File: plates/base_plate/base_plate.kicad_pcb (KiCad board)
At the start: 2 copper layers, 135.6 x 97.4 mm, 0 parts

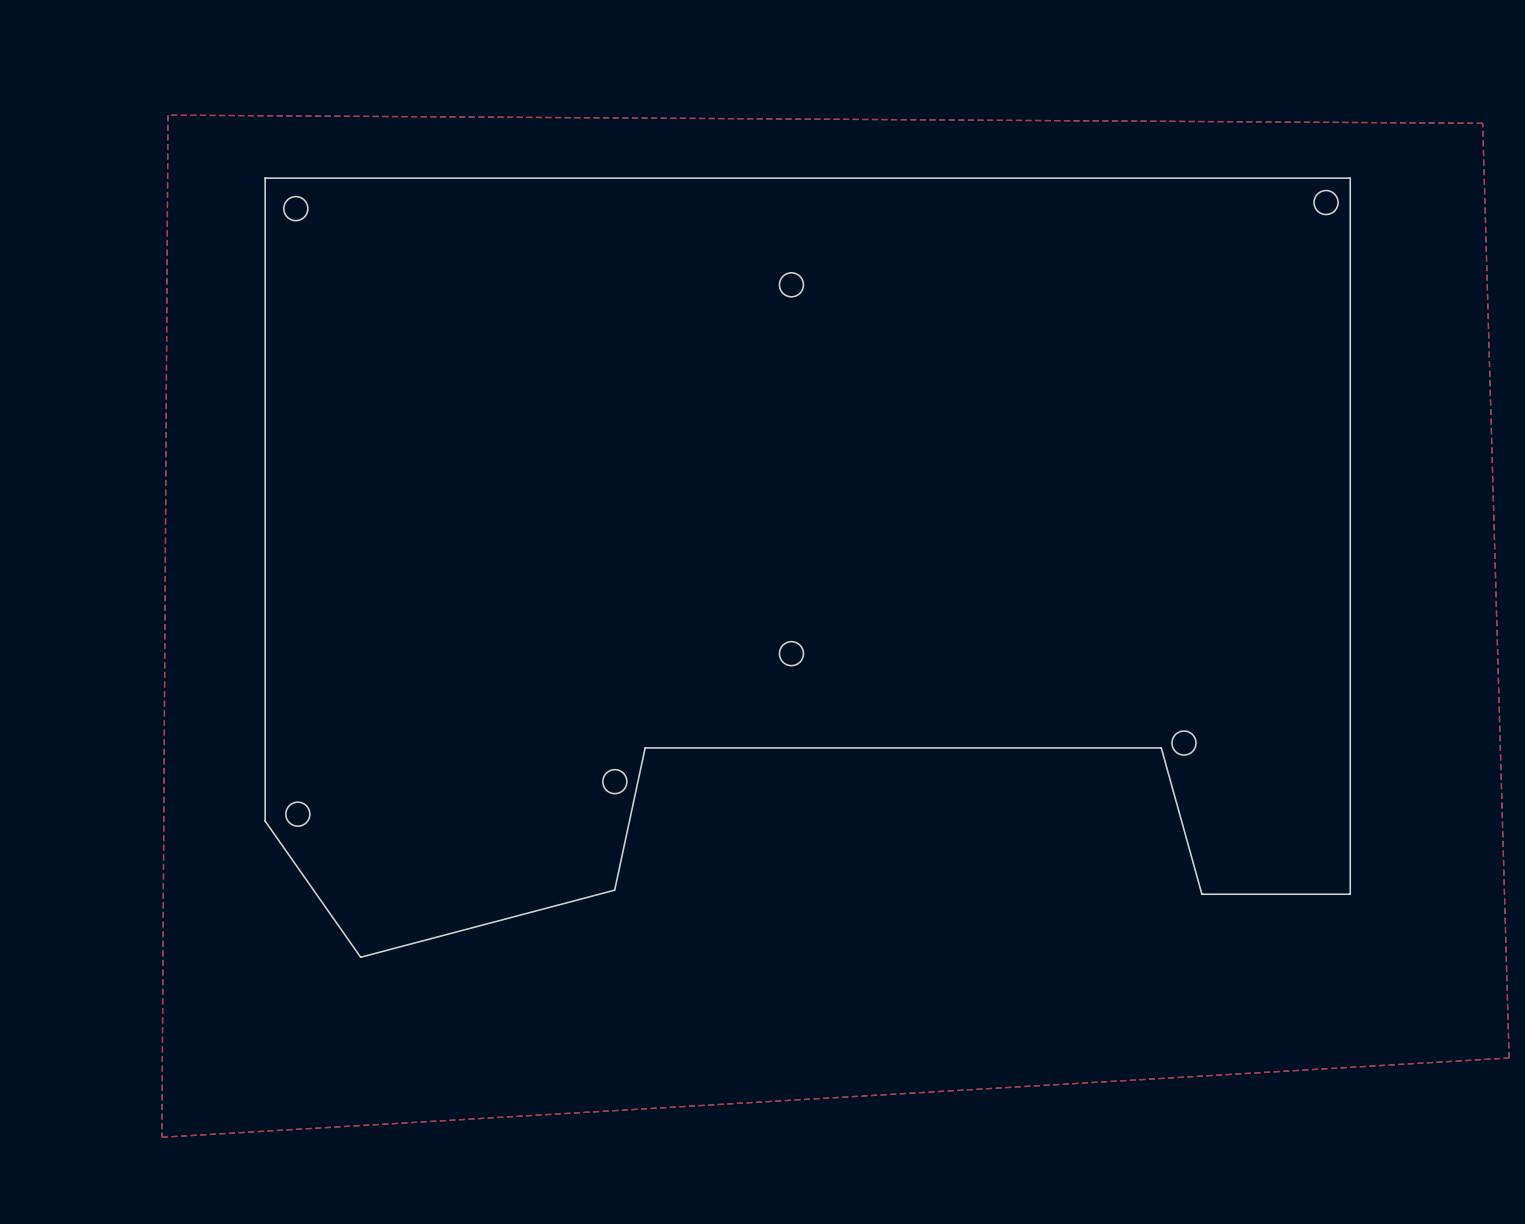
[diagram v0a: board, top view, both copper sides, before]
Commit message: commiting changes before change of name
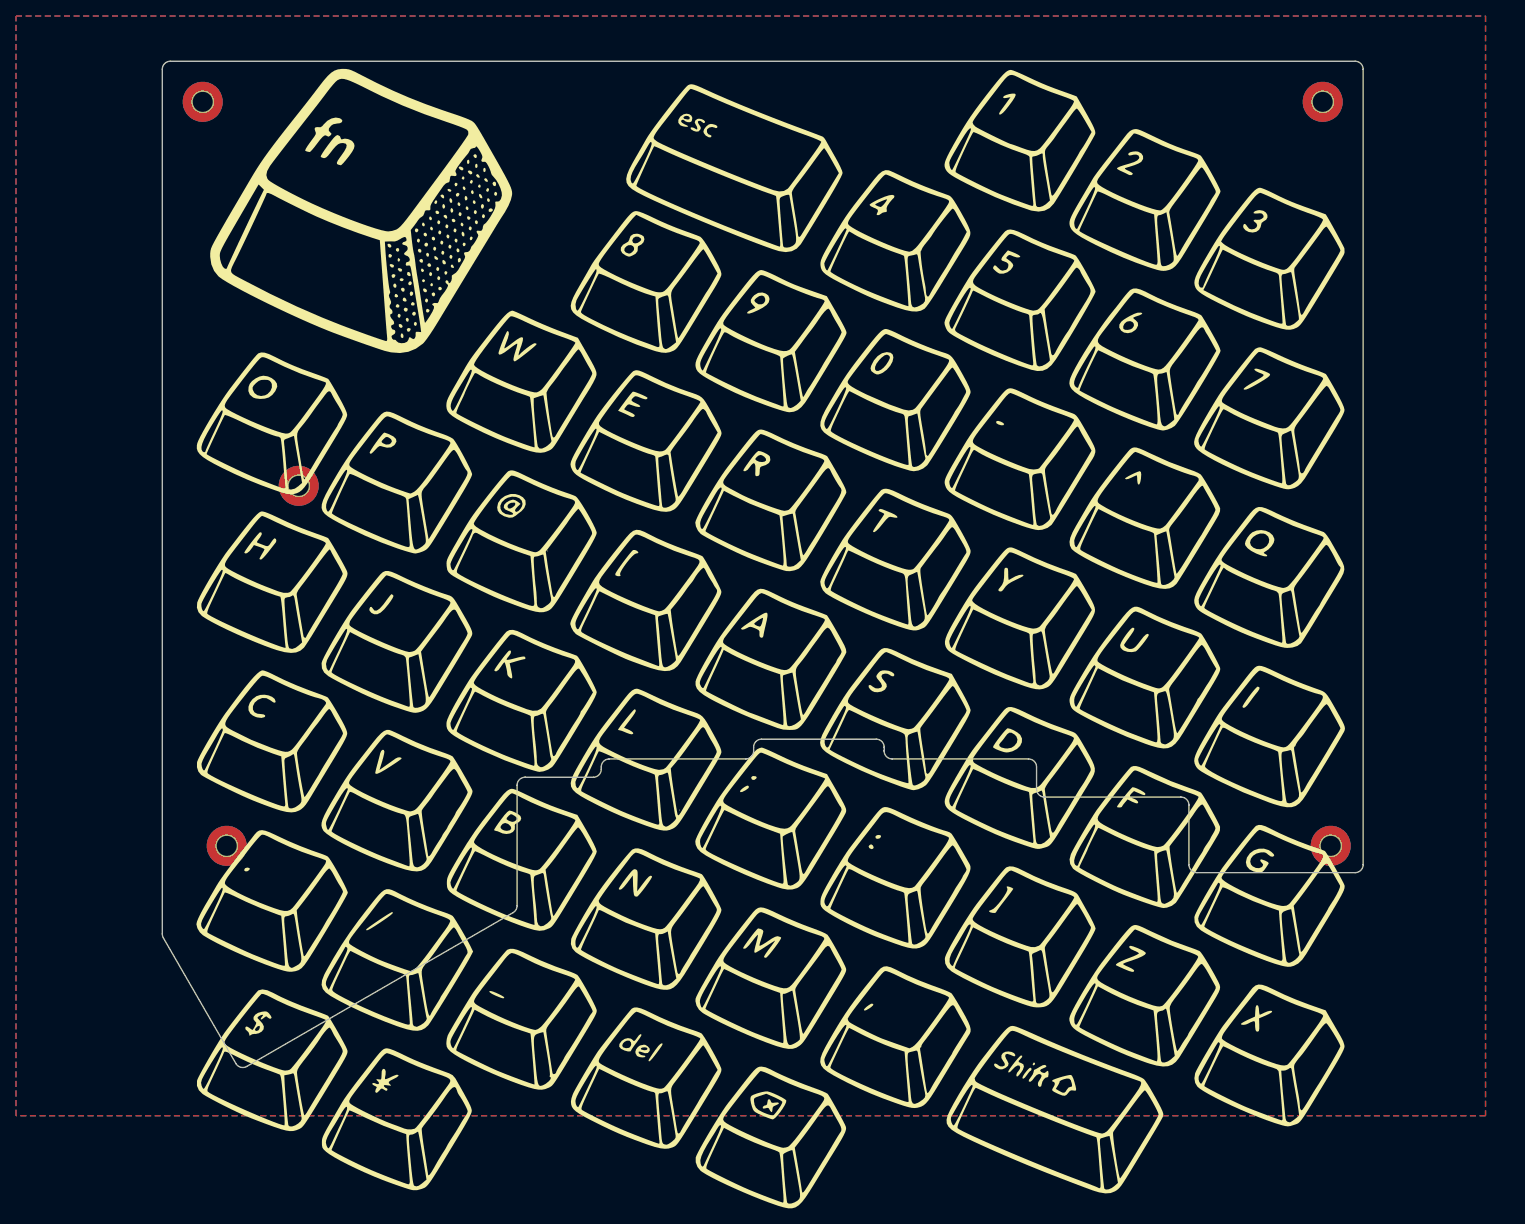
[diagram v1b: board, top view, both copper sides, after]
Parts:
- added G***: LOGO, LOGO, F.Cu at (144.4, 103.2)
- added G***: LOGO, LOGO, B.Cu at (142.9, 103.1)
- added REF**: MountingHole_2.5mm_Pad_TopBottom, MountingHole:MountingHole_2.5mm_Pad_TopBottom, F.Cu at (85.2, 84.7)
- added REF**: MountingHole_2.5mm_Pad_TopBottom, MountingHole:MountingHole_2.5mm_Pad_TopBottom, F.Cu at (73.2, 36.7)
- added REF**: MountingHole_2.5mm_Pad_TopBottom, MountingHole:MountingHole_2.5mm_Pad_TopBottom, F.Cu at (213.2, 36.7)
- added REF**: MountingHole_2.5mm_Pad_TopBottom, MountingHole:MountingHole_2.5mm_Pad_TopBottom, F.Cu at (214.2, 129.7)
- added REF**: MountingHole_2.5mm_Pad_TopBottom, MountingHole:MountingHole_2.5mm_Pad_TopBottom, F.Cu at (76.2, 129.7)
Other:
- board size 135.6 x 97.4 mm -> 150.1 x 125.8 mm
